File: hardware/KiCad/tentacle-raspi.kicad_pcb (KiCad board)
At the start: 2 copper layers, 65 x 56.5 mm, 37 parts, among them P101 CONN_01X06, P102 CONN_01X06, P201 BNC, P301 BNC, P401 BNC

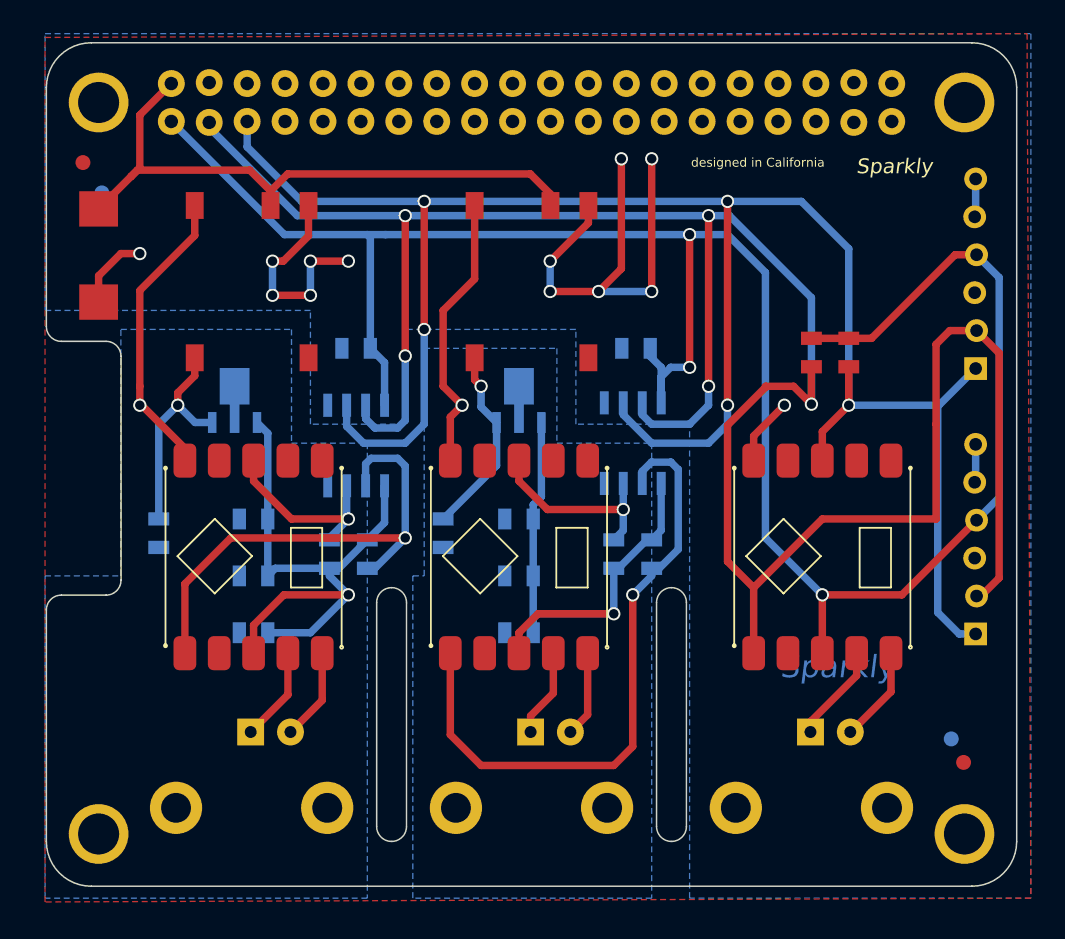
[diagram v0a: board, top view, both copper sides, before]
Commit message: Version 2.0
1wire sensor
flow sensor
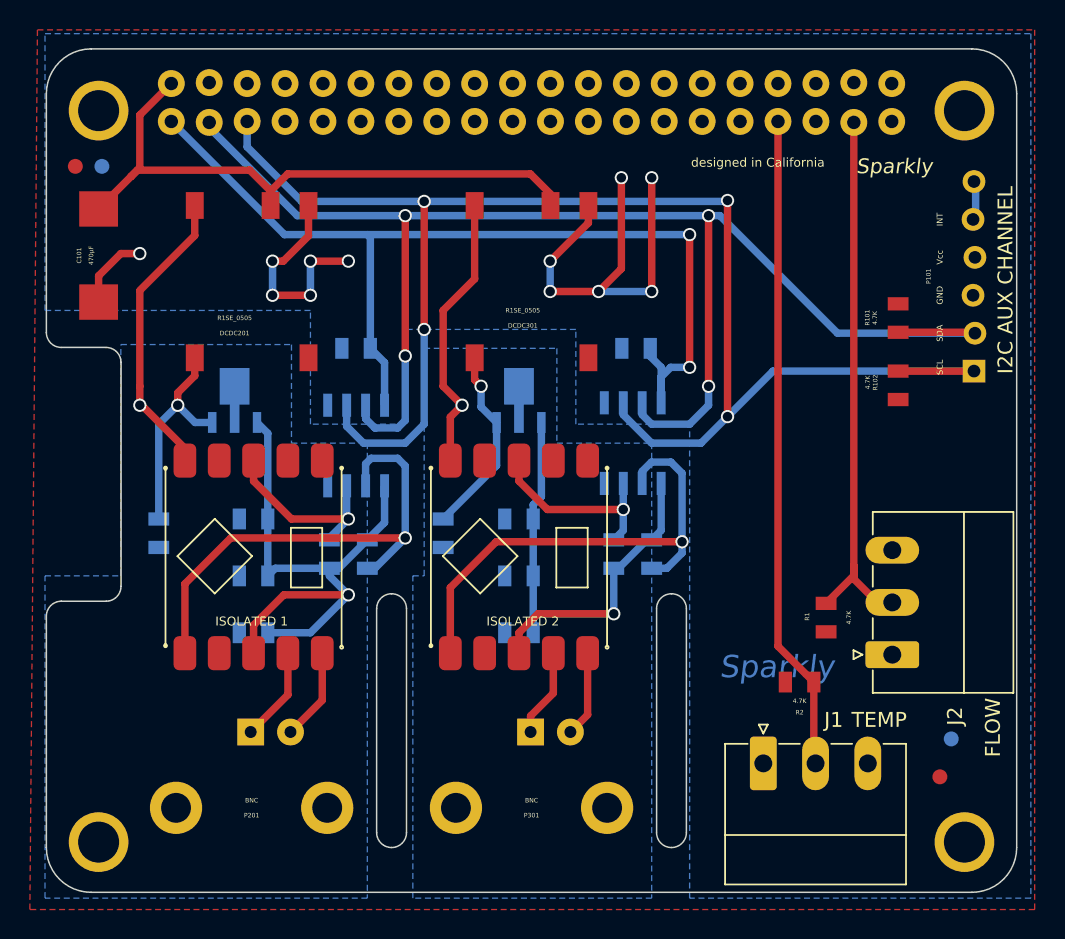
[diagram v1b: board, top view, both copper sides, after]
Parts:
- removed P102: CONN_01X06, temp_terminal:WL-PINH_1X6_snk
- removed P401: BNC, temp_terminal:WL-EB08040502_snk
- removed STP401: EZO_SMD, temp_terminal:WL-ezo-smd
- added J1: Conn_01x03, Connector_Phoenix_MC:PhoenixContact_MC_1,5_3-G-3.5_1x03_P3.50mm_Horizontal, F.Cu at (153.5, 105.3)
- added J2: Conn_01x03, Connector_Phoenix_MC:PhoenixContact_MC_1,5_3-G-3.5_1x03_P3.50mm_Horizontal, F.Cu at (162.2, 98.0)
- added R1: 4.7K, temp_terminal:WL-SM0805R, F.Cu at (157.7, 95.5)
- added R2: 4.7K, temp_terminal:WL-SM0805R, F.Cu at (156.0, 99.8)
- moved R101 6.25 mm to (162.6, 75.4)
- moved R102 3.97 mm to (162.6, 79.9), turned to -90 degrees
- moved fiducial 1.86 mm to (165.4, 106.2)
- moved fiducial 1.78 mm to (109.2, 65.3)
- moved fiducial 0.57 mm to (107.4, 65.3)
- moved PI_Board 0.55 mm to (138.0, 61.5)
- moved P101 0.21 mm to (167.6, 72.6)
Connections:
- PI_BOARD101 pad 33: unconnected-(PI_BOARD101-Pad33) -> /nonisolated1/TEMP
- PI_BOARD101 pad 37: unconnected-(PI_BOARD101-Pad37) -> /nonisolated1/FLOW
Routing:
- net +3.3V: track 144.6 -> 66.5 mm, vias 3 -> 2
- net /SDA: track 162.9 -> 99.0 mm, vias 5 -> 4
- net /nonisolated1/TEMP: track 0.00 -> 44.0 mm
- net /nonisolated1/FLOW: track 0.00 -> 36.5 mm
- net /SCL: track 135.3 -> 104.6 mm, vias 5 -> 4
- net Net-(R302-Pad2): track 42.9 -> 33.0 mm
- net GND: track 56.5 -> 49.4 mm, vias 13 -> 12
- net Net-(P401-Pad1): track 6.56 -> 0.00 mm
- net Net-(P401-Pad2): track 6.43 -> 0.00 mm
- net Net-(P102-Pad5): track 2.57 -> 0.00 mm
- added copper zone on F.Cu, net +3.3V
- removed copper zone on F.Cu, net GND
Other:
- board text added: "FLOW"
- board text added: "I2C AUX CHANNEL"
- board text added: "TEMP"
- board text removed: "CHANNEL 3"
- board text removed: "CHANNEL 4"
- board text removed: "CHANNEL 5"
- board text removed: "NON ISOLATED"
